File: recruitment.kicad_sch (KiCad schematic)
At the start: 3 parts, among them K1 Relay_SPST-NO, U1 ACS781xLRTR-050B

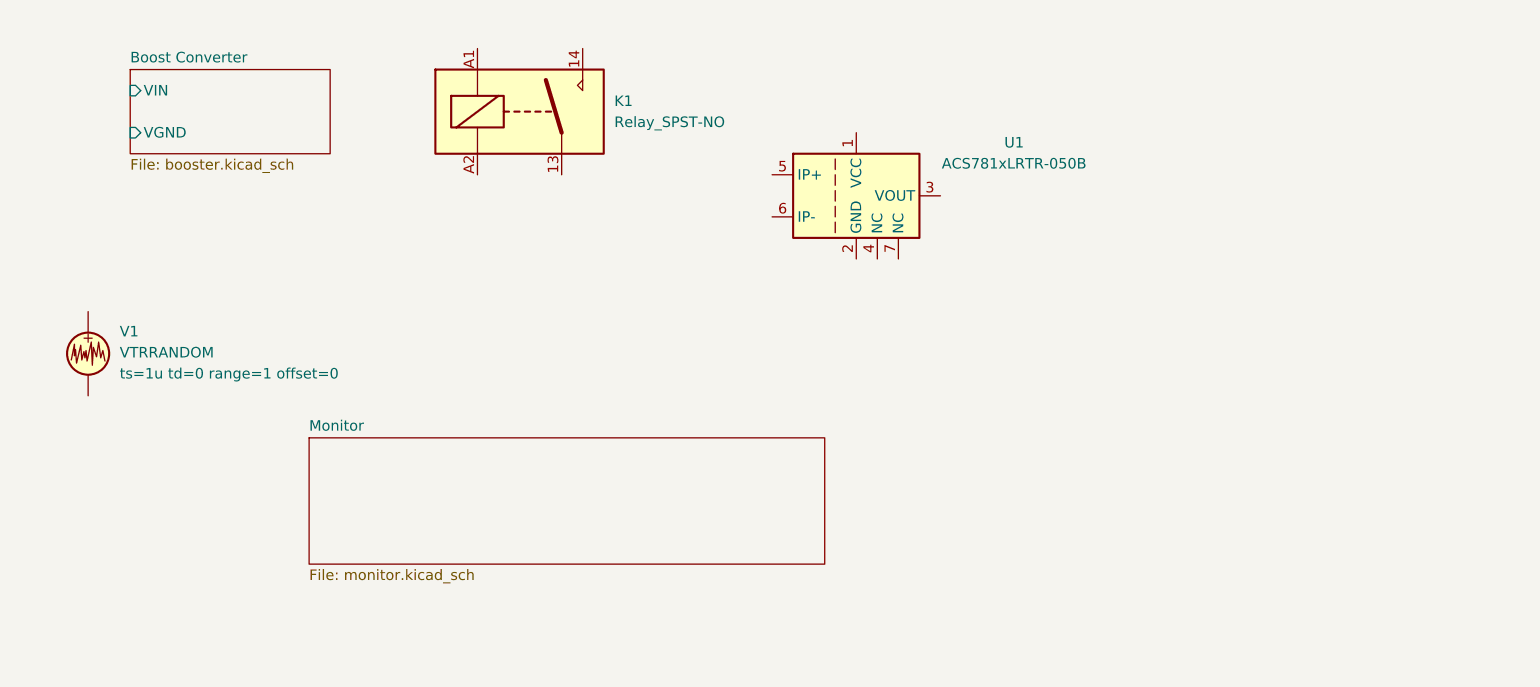
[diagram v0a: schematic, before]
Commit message: partial wiring and monitor draft
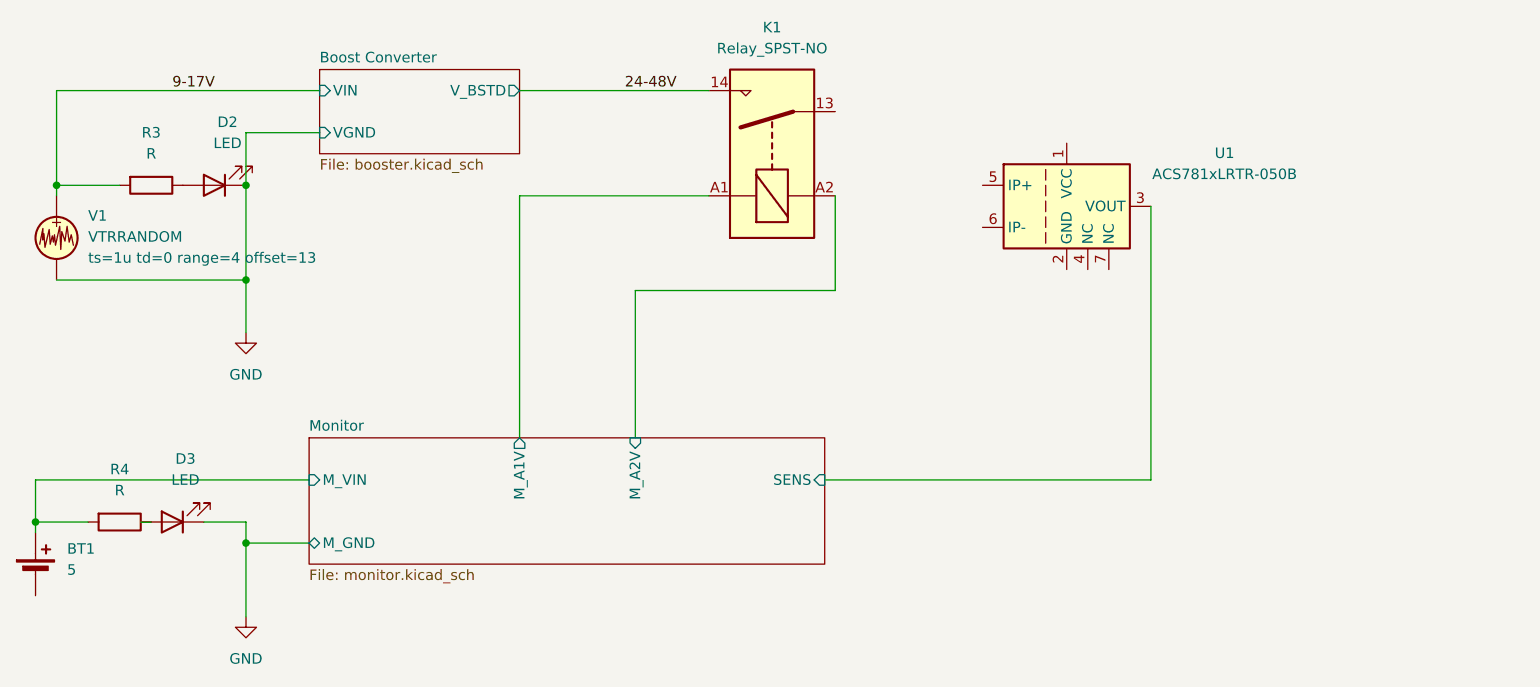
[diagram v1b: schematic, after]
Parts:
- added BT1: 5, symbol Device:Battery_Cell
- added D2, D3: LED, LED_THT:LED_D3.0mm, symbol Device:LED
- added R3, R4: R, symbol Device:R
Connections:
- net Monitor/SENS: now reaches U1.3 (VOUT)
- net 24-48V: now reaches K1.14
- net Monitor/M_A1V: now reaches K1.A1
- net Monitor/M_A2V: now reaches K1.A2
- net 9-17V: now reaches V1.1
- net 9-17V: now also R3.2
- net GND: now reaches V1.2
- net GND: now also D2.1 (K), D3.1 (K)
- new net: D2.2 (A), R3.1
- new net: D3.2 (A), R4.1
- new net Monitor/M_VIN: BT1.1 (+), R4.2
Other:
- sheet Boost Converter ports: added V_BSTD; removed none
- sheet Monitor ports: added M_A1V, M_A2V, M_GND, M_VIN, SENS; removed none
- moved on the sheet: K1, U1, V1

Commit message: monitor changes
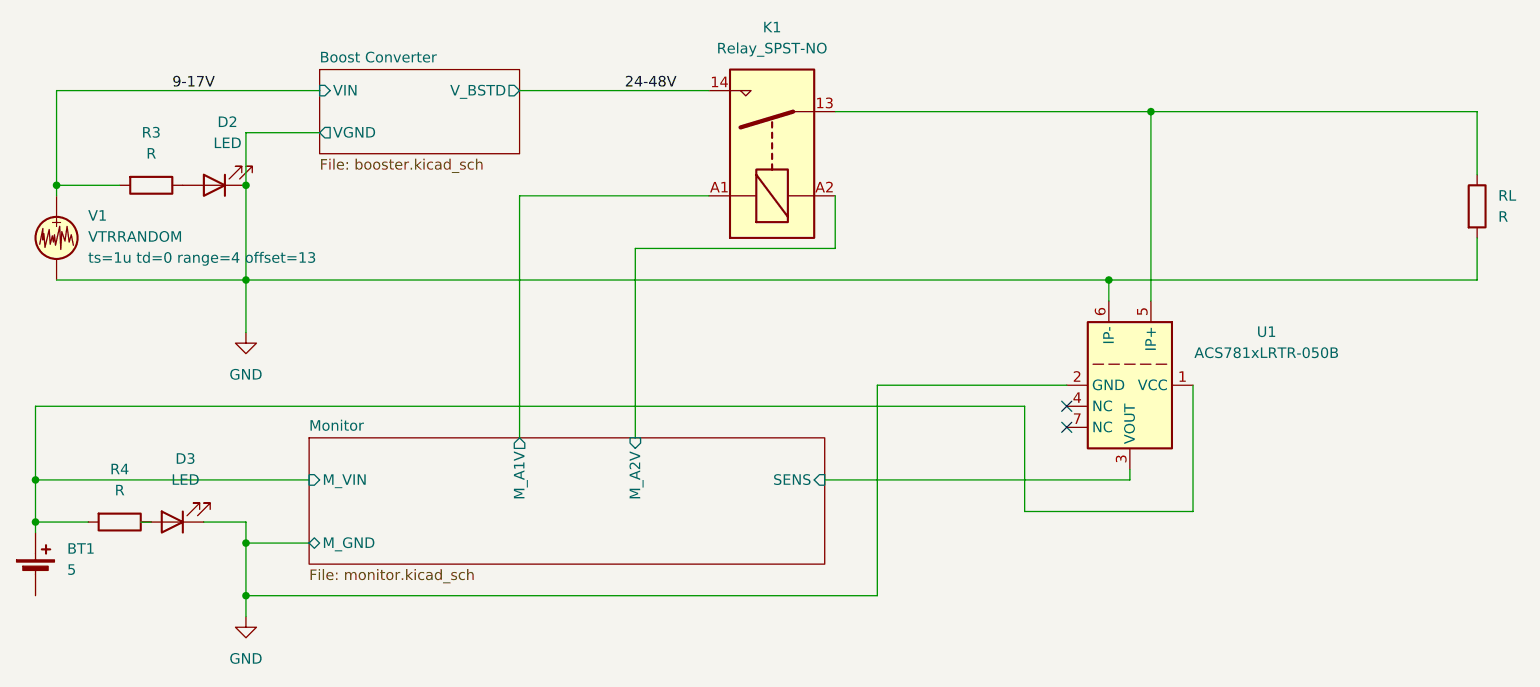
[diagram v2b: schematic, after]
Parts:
- added RL: R, symbol Device:R
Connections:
- net GND: now also U1.2 (GND), U1.6 (IP-), RL.2
- net Monitor/M_VIN: now also U1.1 (VCC)
- net at U1.5 (IP+): now also K1.13, RL.1
- no-connect marks 0 -> 2
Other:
- moved on the sheet: U1
